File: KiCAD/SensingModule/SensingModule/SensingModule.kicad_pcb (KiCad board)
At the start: 2 copper layers, 90 x 70 mm, 39 parts, among them J3 TERMISTOR, U1 Arduino MKR WAN 1310, U2 NJM7805SDL1, U3 MCP2562-E-P, U4 MCP2515-I/P, U5 MB85RS2MT, U6 MB85RS2MT, U7 MB85RS2MT, U8 MB85RS2MT, Y1 8MHz

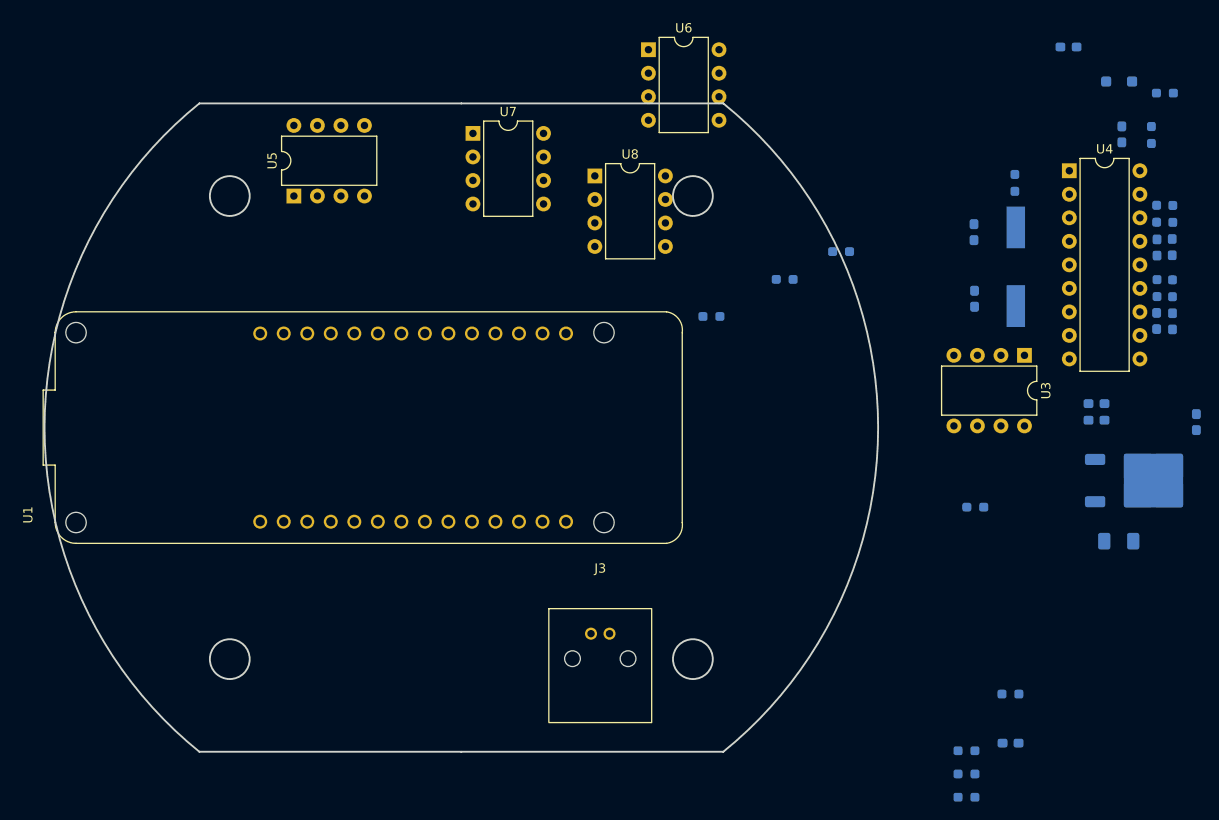
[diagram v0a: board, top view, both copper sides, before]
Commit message: コネクタ以外は基板の中に入った
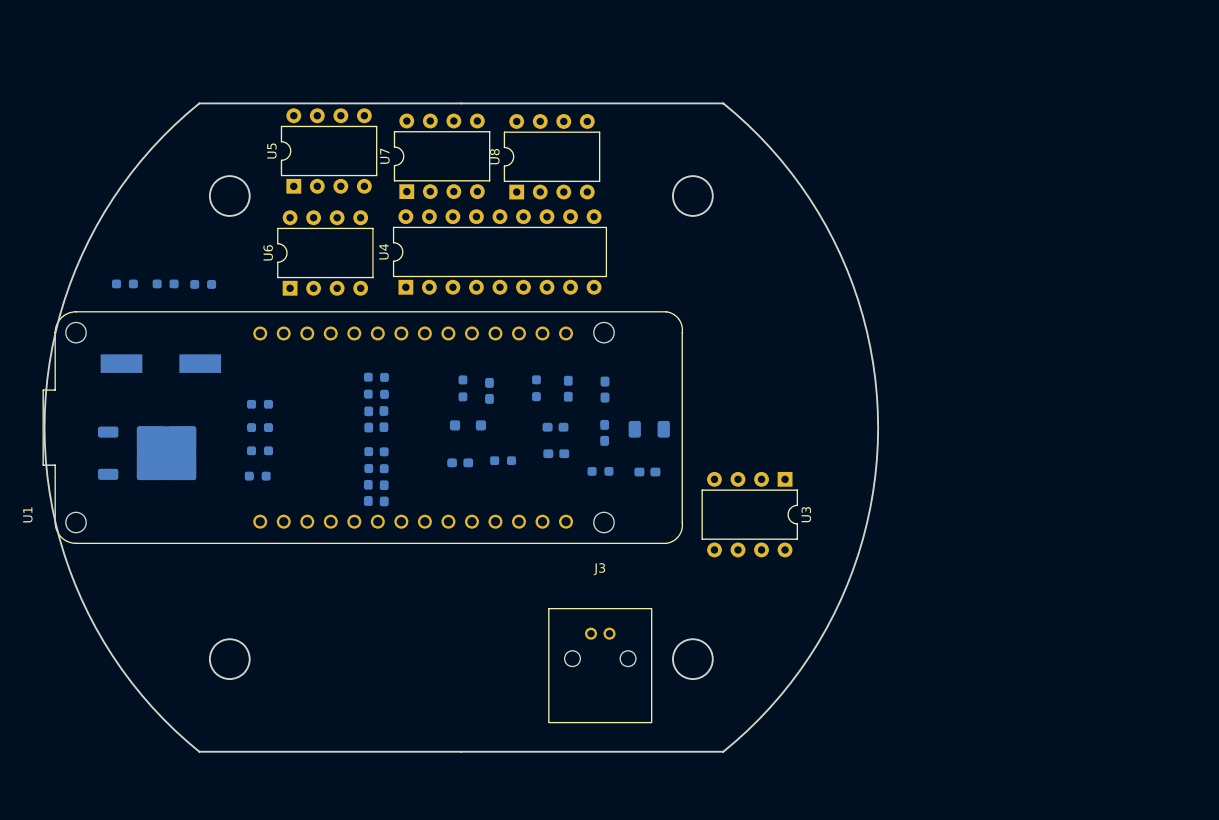
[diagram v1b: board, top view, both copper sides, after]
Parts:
- moved U2 106.6 mm to (116.9, 102.8)
- moved Y1 92.9 mm to (117.6, 93.1), turned to 0 degrees
- moved D1 87.1 mm to (141.6, 99.1)
- moved D2 87.1 mm to (140.0, 99.1)
- moved D5 87.1 mm to (141.7, 107.1)
- moved R1 87.1 mm to (141.7, 95.5)
- moved R7 87.1 mm to (141.7, 103.5)
- moved R8 87.1 mm to (140.0, 103.5)
- moved D6 87.1 mm to (140.0, 107.1)
- moved R2 87.1 mm to (140.0, 95.5)
- moved R13 85.0 mm to (128.3, 100.0)
- moved R12 85.0 mm to (128.3, 97.5)
- moved R14 85.0 mm to (128.3, 102.5)
- moved R10 81.7 mm to (154.5, 103.6)
- moved D3 79.6 mm to (149.9, 103.8)
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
